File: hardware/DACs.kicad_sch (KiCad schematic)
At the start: 52 parts, among them J6 Conn_Coaxial, J7 Conn_Coaxial, J8 Conn_Coaxial, J9 Conn_Coaxial, U10 LTC2642, U11 LTC2642, U12 REF35250QDBVR, U4 OPA2994IDGKR, U5 OPA2994IDGKR, U6 OPA2994IDGKR, U7 OPA2994IDGKR, U8 LTC2642, U9 LTC2642

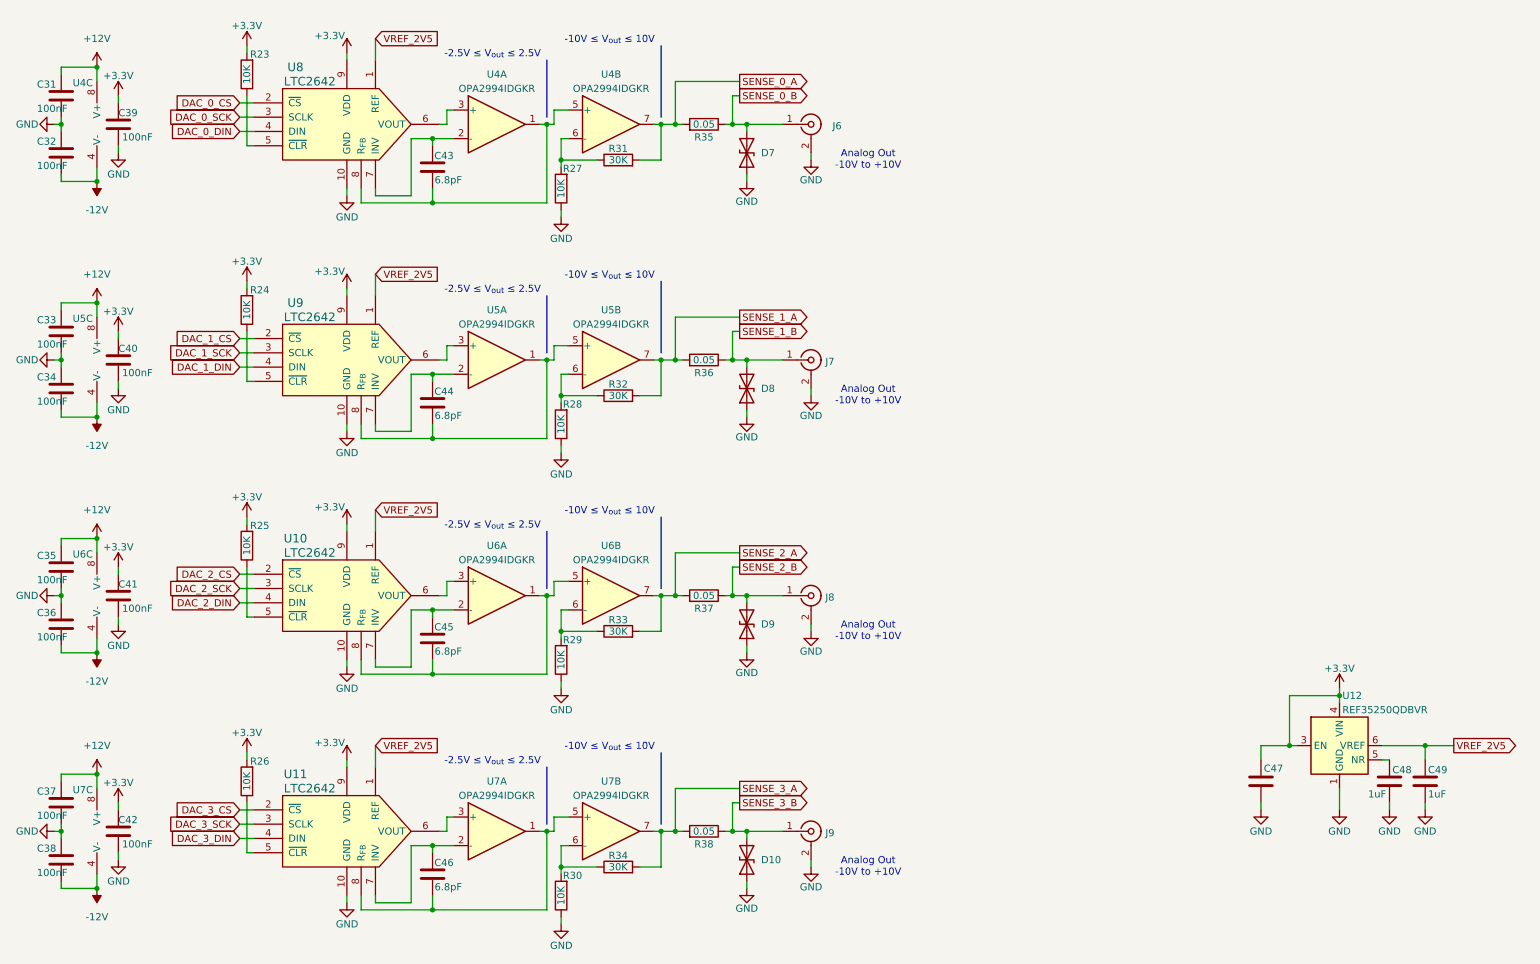
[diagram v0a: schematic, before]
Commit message: update pcb
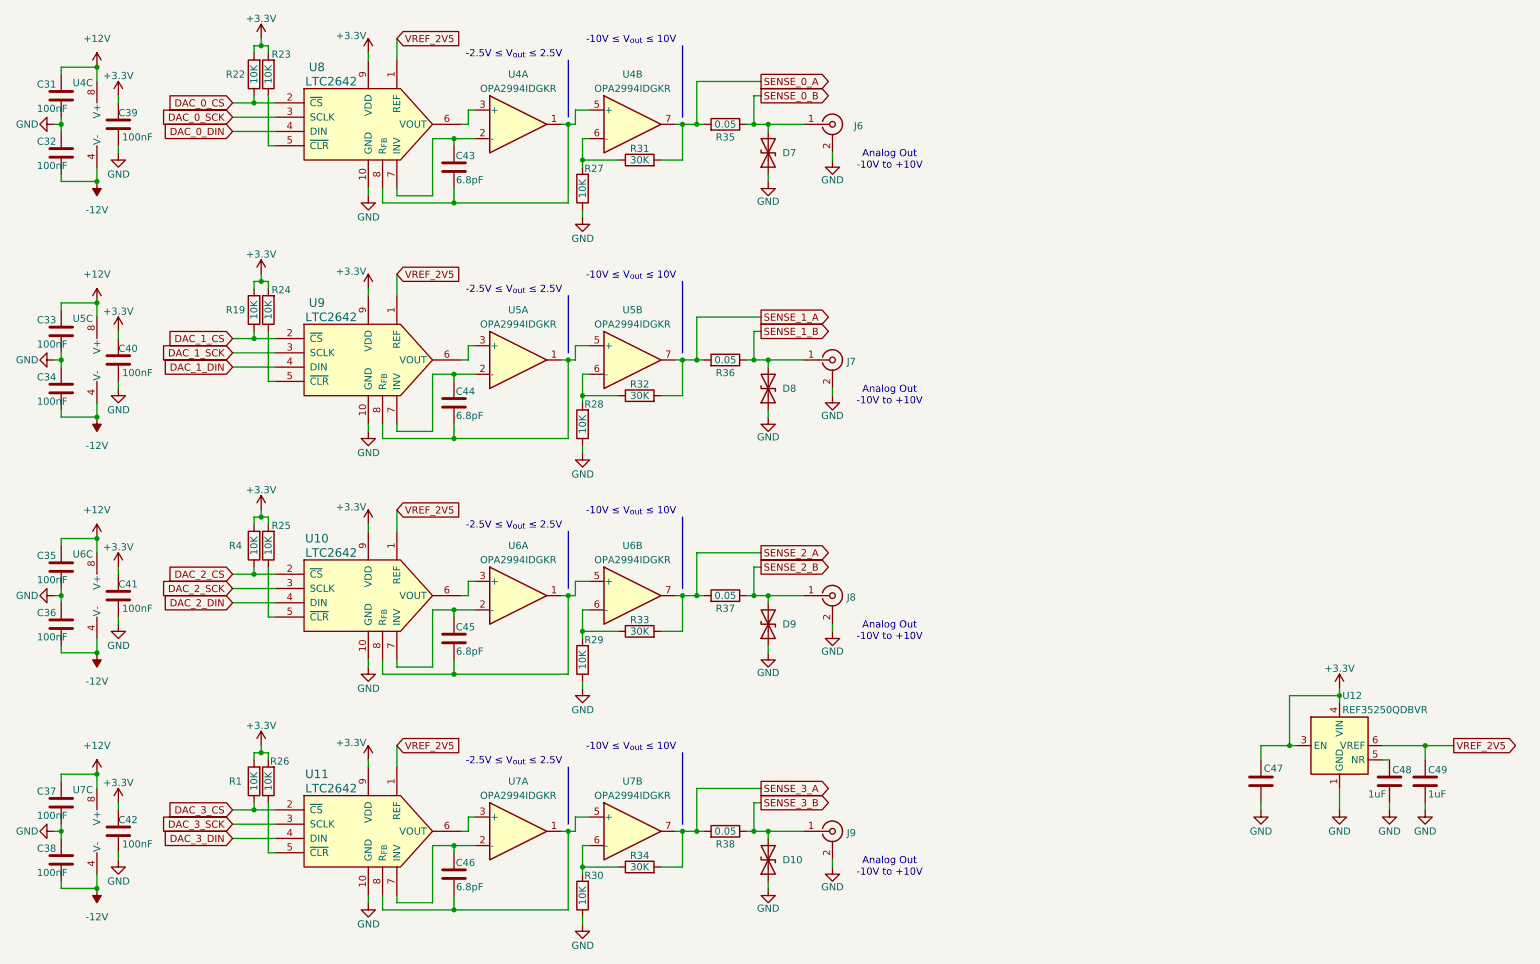
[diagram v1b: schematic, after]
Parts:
- added R1, R19, R22, R4: 10K, Resistor_SMD:R_0402_1005Metric, symbol Device:R
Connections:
- net +3.3V: now also R1.2, R19.2, R22.2, R4.2
- net DAC_0_CS: now also R22.1
- net DAC_1_CS: now also R19.1
- net DAC_2_CS: now also R4.1
- net DAC_3_CS: now also R1.1
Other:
- moved on the sheet: C43, C44, C45, C46, D10, D7, D8, D9, J6, J7, J8, J9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
